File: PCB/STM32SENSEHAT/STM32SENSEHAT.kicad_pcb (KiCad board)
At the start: 2 copper layers, 74 parts, among them J1 USB_B_Micro, J10 Conn_01x01_Pin, J11 Conn_01x02_Pin, J2 Conn_01x05_Pin, J5 Conn_01x24_Pin, J8 Conn_01x24_Pin, J9 Conn_01x10_Pin, Q1 FS8205A, SW1 SW_Push, U1 MCP1700x-330xxTT, U11 AO3401A_C306862, U3 FT234XD-R, U4 TMP102xxDRL, U5 CAT24C256, U6 LTR-303ALS-01, U9 STLINK_UCT

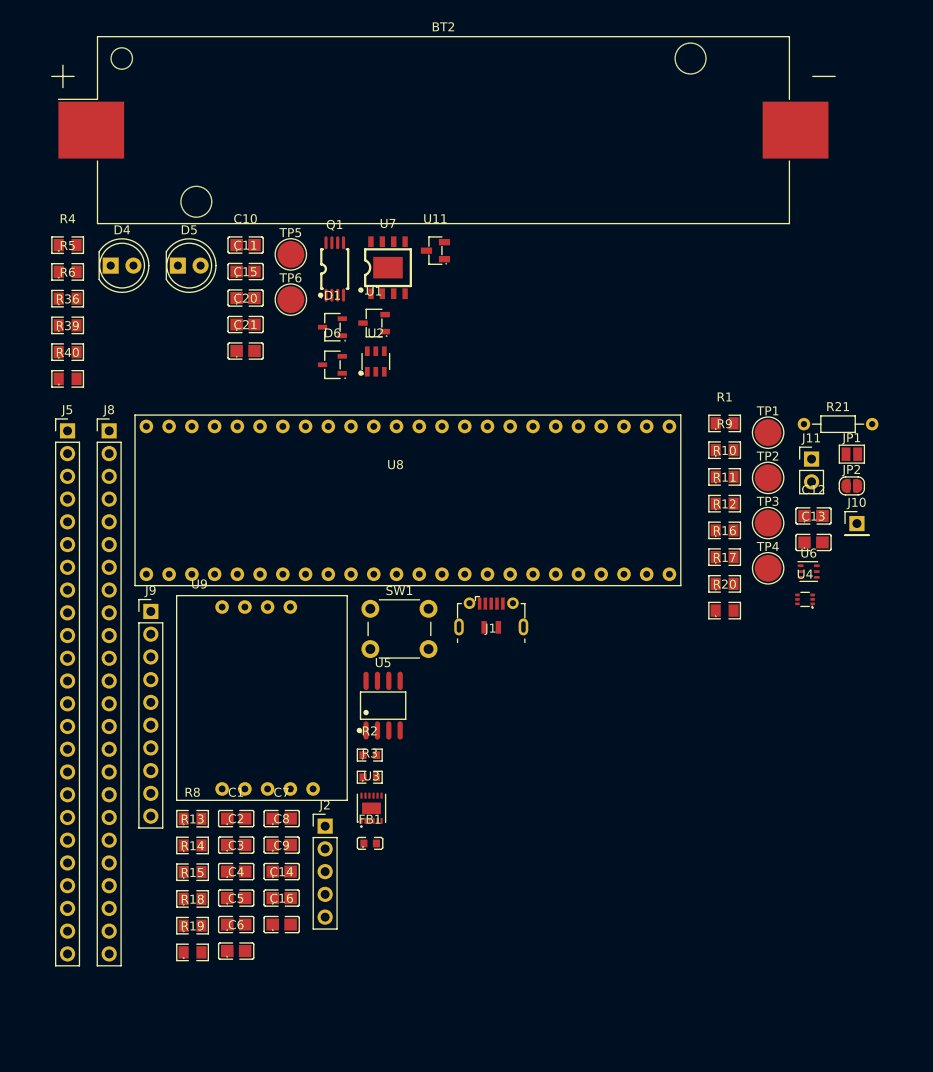
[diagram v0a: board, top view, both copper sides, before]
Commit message: PCB draft
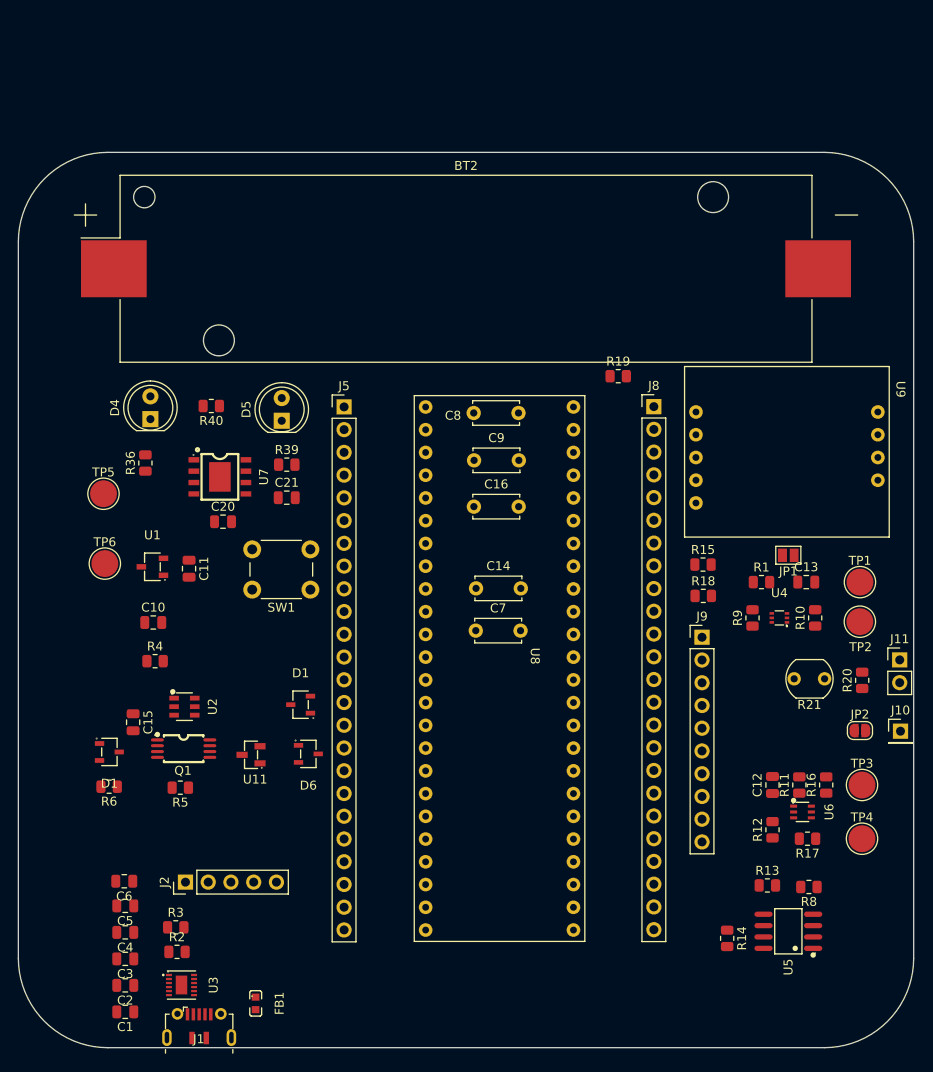
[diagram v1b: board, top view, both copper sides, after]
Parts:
- added D1: D_Schottky, JLCfootprint:SOT-23-3_L3.0-W1.7-P0.95-LS2.9-BR, F.Cu at (110.2, 107.0)
- C1, C10, C11, C12, C13, C15, C2, C20, C21, C3, C4, C5, C6: footprint JLCfootprint:C0805 -> Capacitor_SMD:C_0805_2012Metric
- C14, C16, C7, C8, C9: footprint JLCfootprint:C0805 -> Capacitor_THT:C_Disc_D5.0mm_W2.5mm_P5.00mm
- R1, R10, R11, R12, R13, R14, R15, R16, R17, R18, R19, R20, R36, R39, R4, R40, R5, R6, R8, R9: footprint JLCfootprint:R0805 -> Resistor_SMD:R_0805_2012Metric
- R2, R3: footprint JLCfootprint:R0603 -> Resistor_SMD:R_0805_2012Metric
- R21: footprint Resistor_THT:R_Axial_DIN0204_L3.6mm_D1.6mm_P7.62mm_Horizontal -> OptoDevice:R_LDR_5.1x4.3mm_P3.4mm_Vertical
- U2: value ~ -> DW01A
- U6: footprint OptoDevice:Lite-On_LTR-303ALS-01 -> JLCfootprint:SOT-363_L2.0-W1.3-P0.65-LS2.1-BL
- U7: value ~ -> TP4056
- moved R19 80.0 mm to (167.0, 65.0)
- moved R8 69.3 mm to (188.3, 122.0), turned to 180 degrees
- moved R15 68.2 mm to (176.5, 86.0)
- moved R18 67.9 mm to (176.5, 89.5)
- moved U9 65.6 mm to (185.8, 72.8), turned to -90 degrees
- moved R13 64.4 mm to (183.7, 121.9)
- moved J9 61.6 mm to (176.4, 94.2)
- moved J8 60.9 mm to (171.0, 68.4)
- moved R14 60.2 mm to (179.2, 127.8), turned to -90 degrees
- moved U11 60.0 mm to (126.0, 107.3)
- moved R5 59.0 mm to (118.1, 111.0), turned to 180 degrees
- moved J1 56.3 mm to (120.1, 139.5)
- moved Q1 56.2 mm to (118.5, 106.6), turned to -90 degrees
- moved R6 54.7 mm to (110.1, 110.8), turned to 180 degrees
- moved C8 52.8 mm to (150.9, 69.1)
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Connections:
- BT2 pad 1: /POWER MANAGEMENT MODULE/BATT+ -> Net-(BT2-+)
- C15 pad 2: Net-(D1-K) -> Net-(BT2--)
- Q1 pad 2: Net-(D1-K) -> Net-(BT2--)
- Q1 pad 3: Net-(D1-K) -> Net-(BT2--)
- U2 pad 6: Net-(D1-K) -> Net-(BT2--)
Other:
- board outline added: 100 x 100 mm
